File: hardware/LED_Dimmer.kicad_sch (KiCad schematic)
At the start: 11 parts, among them J1 Molex PicoBlade 53261-0871 1x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, Q1 2N7002K-7, Q2 2N7002K-7, Q3 2N7002K-7, U1 BGM220P, U2 L78L33A

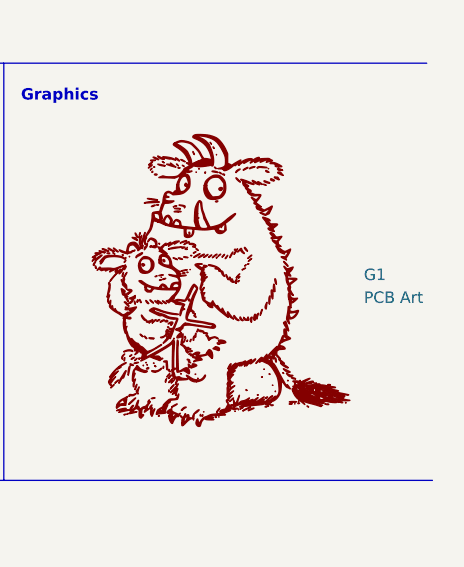
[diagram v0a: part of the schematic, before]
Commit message: Changed a digikey PN and removed the gruffalo art from the BOM
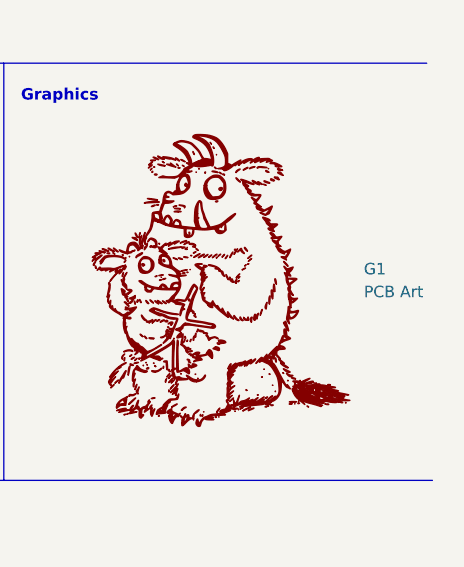
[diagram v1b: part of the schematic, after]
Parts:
- U2: Digikey PN L78L33ACD-ND -> 497-1199-1-ND
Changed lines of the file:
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@@
       (effects (font (size 1.27 1.27)) hide)
     )
-    (property "Digikey PN" "L78L33ACD-ND" (at 50.8 137.16 0)
+    (property "Digikey PN" "497-1199-1-ND" (at 50.8 137.16 0)
       (effects (font (size 1.27 1.27)) hide)
     )
@@
   (symbol (lib_id "Gruffalo_Dimmer:PCB Art") (at 262.255 88.9 0) (unit 1)
     (in_bom no) (on_board yes) (dnp no) (fields_autoplaced)
-    (property "Reference" "G1" (at 278.13 88.2783 0)
-      (effects (font (size 1.27 1.27)) (justify left))
-    )
-    (property "Value" "PCB Art" (at 278.13 90.8183 0)
-      (effects (font (size 1.27 1.27)) (justify left))
-    )
+    (property "Reference" "G1" (at 278.13 87.6433 0)
+      (effects (font (size 1.27 1.27)) (justify left))
+    )
+    (property "Value" "PCB Art" (at 278.13 90.1833 0)
+      (effects (font (size 1.27 1.27)) (justify left))
+    )
